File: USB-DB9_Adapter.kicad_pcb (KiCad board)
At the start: 2 copper layers, 31.3 x 30.2 mm, 41 parts, among them IC2 STM32G0B1KBU6-N, U2 U_SPANNUNGSREGLERSOT23, X1 USB-1X-2S-PLUG-A-SMD, X4 M09H, X7 SWD_MOSER_CONN_5_POLST

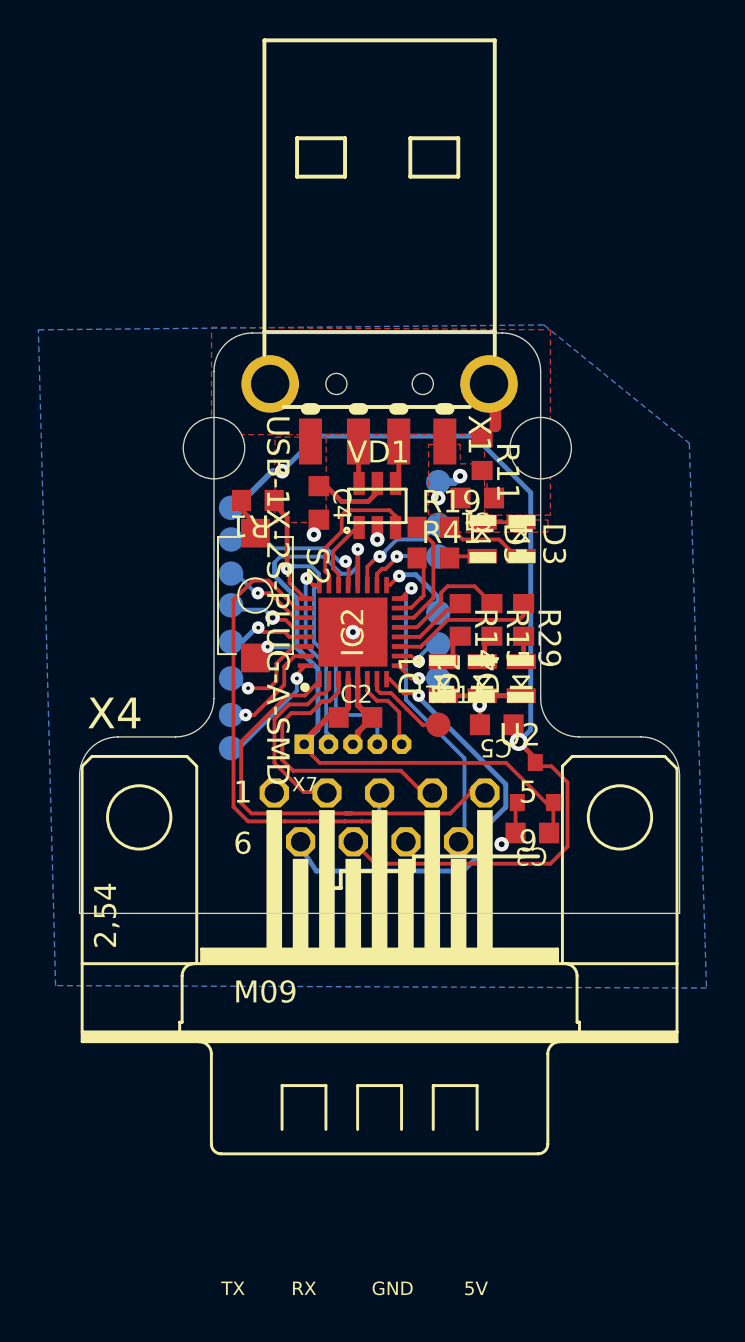
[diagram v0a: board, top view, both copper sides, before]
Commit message: Add files via upload
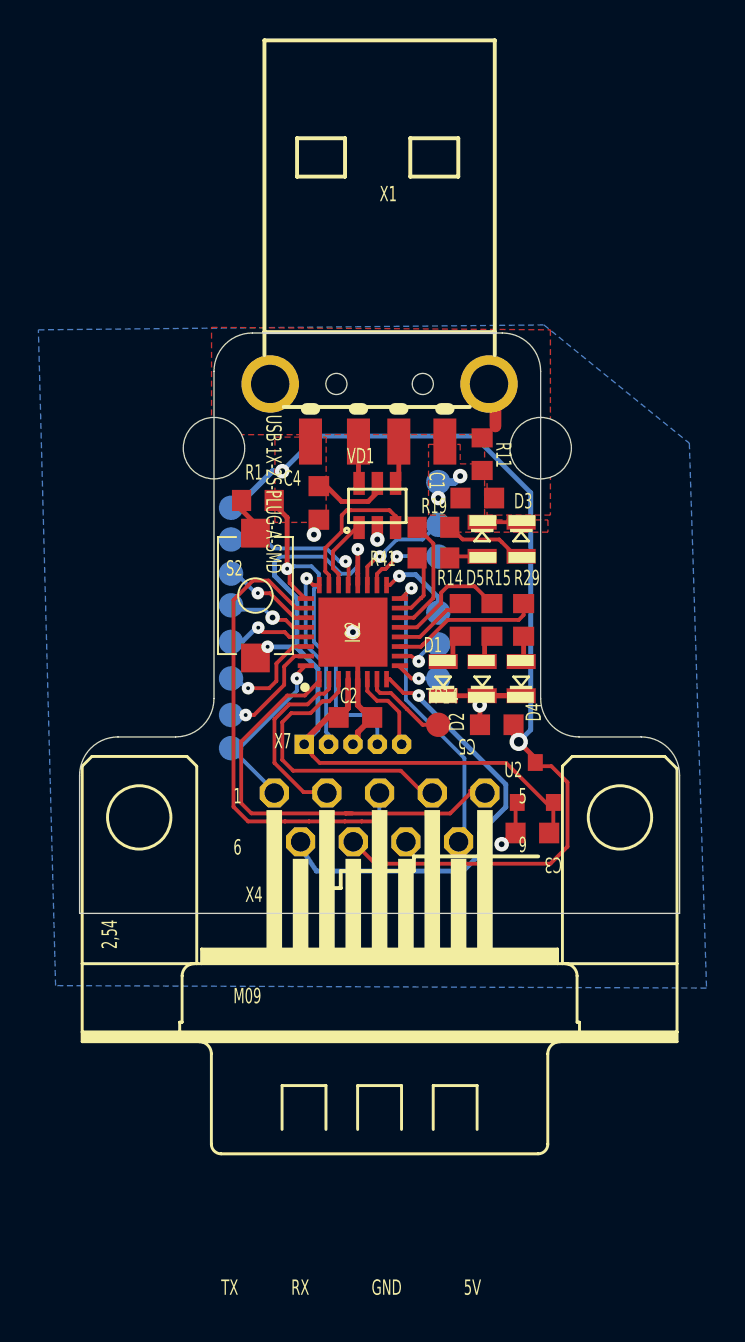
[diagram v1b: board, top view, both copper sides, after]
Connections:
- IC2 pad 32: Net-(IC2-PB8) -> /UP
- TP3 pad TP: Net-(IC2-PB8) -> /UP
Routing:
- net /UP: track 0.00 -> 9.42 mm, vias 0 -> 1
- net Net-(IC2-PB8): track 6.15 -> 0.00 mm, vias 1 -> 0
